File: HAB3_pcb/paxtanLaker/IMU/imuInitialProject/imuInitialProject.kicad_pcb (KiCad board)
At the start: 2 copper layers, 12 parts, among them J1 Conn_01x09_Female, J2 Conn_01x02_Female, U1 LSM9DS0

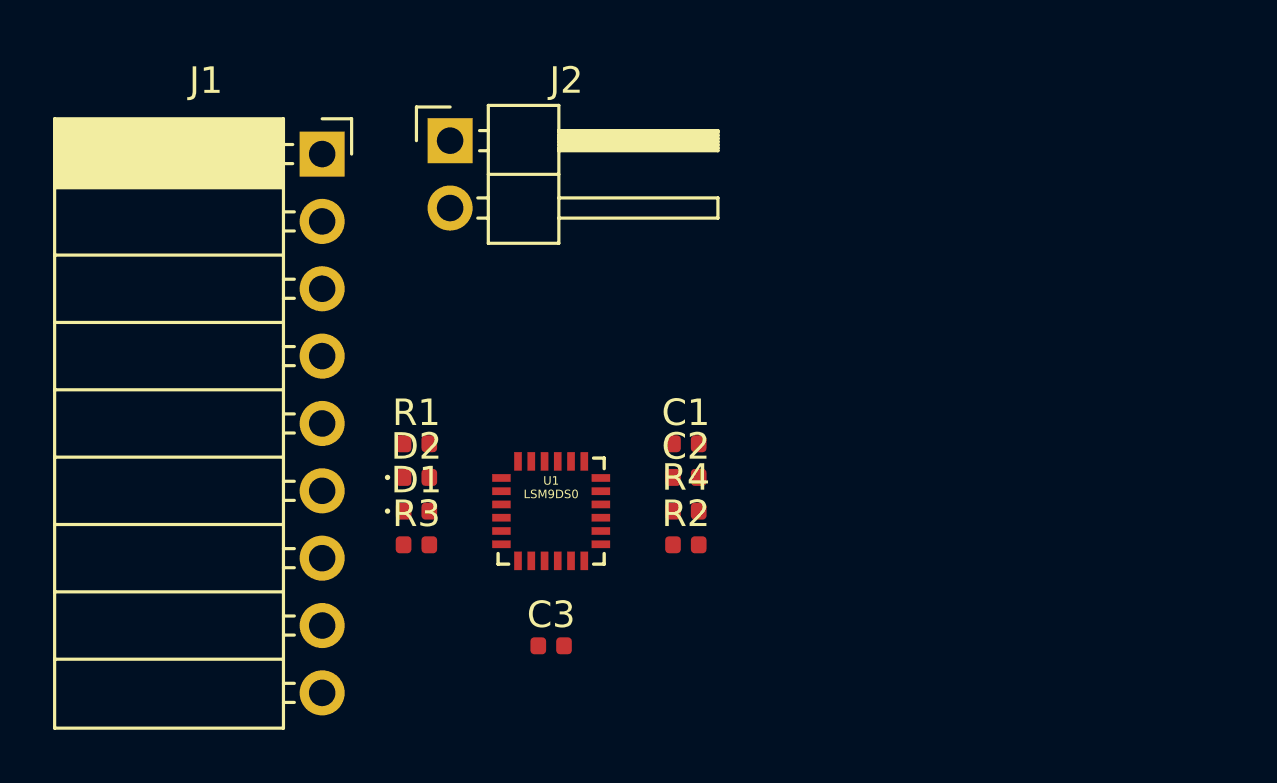
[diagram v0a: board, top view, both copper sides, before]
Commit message: started tracing
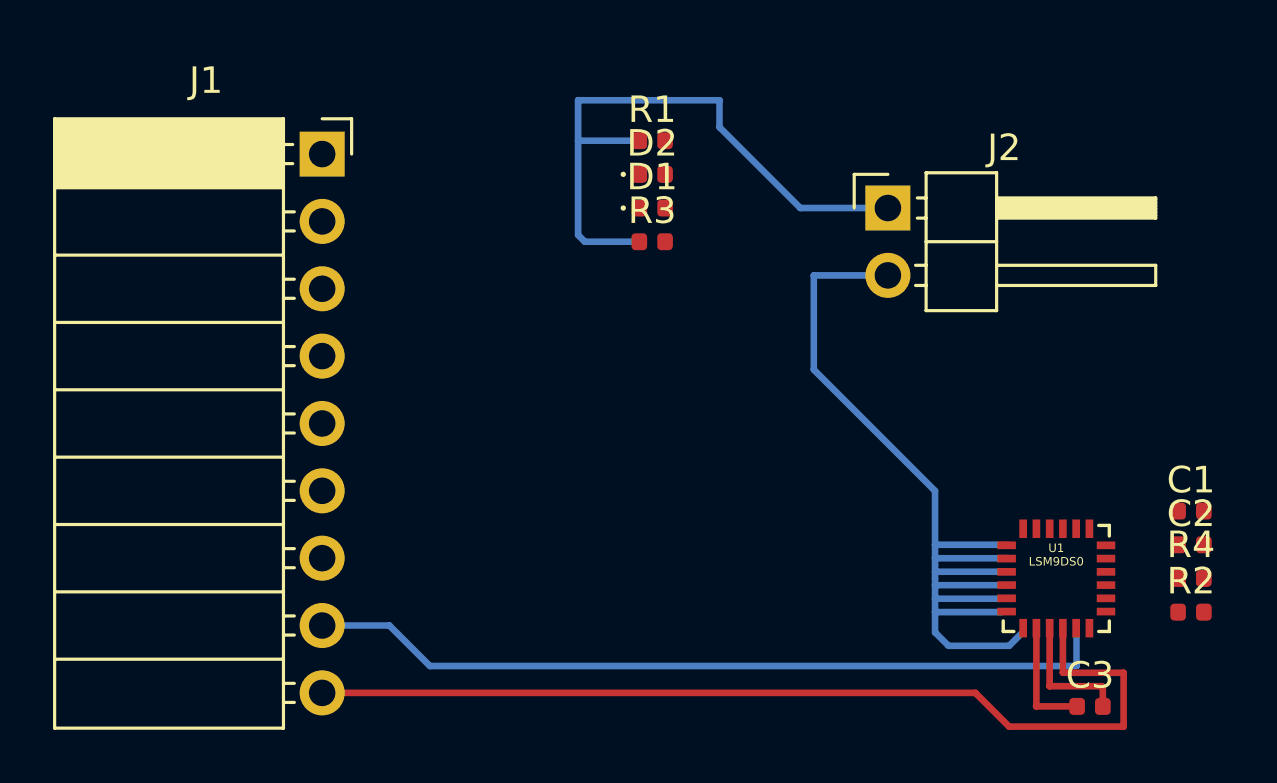
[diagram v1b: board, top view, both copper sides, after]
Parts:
- moved C3 20.4 mm to (167.6, 88.6)
- moved U1 19.2 mm to (166.4, 83.8)
- moved C1 19.2 mm to (171.4, 81.3)
- moved R2 19.2 mm to (171.4, 85.1)
- moved C2 19.2 mm to (171.4, 82.5)
- moved R4 19.2 mm to (171.4, 83.8)
- moved J2 16.7 mm to (160.0, 69.8)
- moved D1 14.5 mm to (151.1, 69.8)
- moved D2 14.5 mm to (151.1, 68.6)
- moved R1 14.5 mm to (151.1, 67.3)
- moved R3 14.5 mm to (151.1, 71.1)
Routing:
- net Net-(C1-Pad1): track 0.00 -> 38.1 mm
- net Net-(J1-Pad9): track 0.00 -> 36.8 mm
- net Net-(J1-Pad8): track 0.00 -> 30.3 mm
- net Net-(C1-Pad2): track 0.00 -> 23.7 mm
- net Net-(C3-Pad2): track 0.00 -> 4.95 mm
- net Net-(C3-Pad1): track 0.00 -> 4.50 mm
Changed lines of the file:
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@@
   (general
     (thickness 1.6)
-    (drawings 4)
-    (tracks 0)
+    (drawings 6)
+    (tracks 49)
     (zones 0)
     (modules 12)
@@
   )
   (module Capacitor_SMD:C_0402_1005Metric (layer F.Cu)
-    (at 152.4 78.74)
+    (at 171.45 81.28)
     (descr "Capacitor SMD 0402 (1005 Metric), square (rectangular) end terminal, IPC_7351 nominal, (Body size source: http://www.tortai-tech.com/upload/download/2011102023233369053.pdf), generated with kicad-footprint-generator")
     (tags capacitor)
@@
   )
   (module Capacitor_SMD:C_0402_1005Metric (layer F.Cu)
-    (at 152.4 80.01)
+    (at 171.45 82.55)
     (descr "Capacitor SMD 0402 (1005 Metric), square (rectangular) end terminal, IPC_7351 nominal, (Body size source: http://www.tortai-tech.com/upload/download/2011102023233369053.pdf), generated with kicad-footprint-generator")
     (tags capacitor)
@@
   )
   (module Capacitor_SMD:C_0402_1005Metric (layer F.Cu)
-    (at 147.32 86.36)
+    (at 167.64 88.646)
     (descr "Capacitor SMD 0402 (1005 Metric), square (rectangular) end terminal, IPC_7351 nominal, (Body size source: http://www.tortai-tech.com/upload/download/2011102023233369053.pdf), generated with kicad-footprint-generator")
     (tags capacitor)
@@
   )
   (module Diode_SMD:D_0402_1005Metric (layer F.Cu)
-    (at 142.24 81.28)
+    (at 151.13 69.85)
     (descr "Diode SMD 0402 (1005 Metric), square (rectangular) end terminal, IPC_7351 nominal, (Body size source: http://www.tortai-tech.com/upload/download/2011102023233369053.pdf), generated with kicad-footprint-generator")
     (tags diode)
@@
   )
   (module Diode_SMD:D_0402_1005Metric (layer F.Cu)
-    (at 142.24 80.01)
+    (at 151.13 68.58)
     (descr "Diode SMD 0402 (1005 Metric), square (rectangular) end terminal, IPC_7351 nominal, (Body size source: http://www.tortai-tech.com/upload/download/2011102023233369053.pdf), generated with kicad-footprint-generator")
     (tags diode)
@@
   )
   (module Resistor_SMD:R_0402_1005Metric (layer F.Cu)
-    (at 142.24 78.74)
+    (at 151.13 67.31)
     (descr "Resistor SMD 0402 (1005 Metric), square (rectangular) end terminal, IPC_7351 nominal, (Body size source: http://www.tortai-tech.com/upload/download/2011102023233369053.pdf), generated with kicad-footprint-generator")
     (tags resistor)
@@
   )
   (module Resistor_SMD:R_0402_1005Metric (layer F.Cu)
-    (at 152.4 82.55)
+    (at 171.45 85.09)
     (descr "Resistor SMD 0402 (1005 Metric), square (rectangular) end terminal, IPC_7351 nominal, (Body size source: http://www.tortai-tech.com/upload/download/2011102023233369053.pdf), generated with kicad-footprint-generator")
     (tags resistor)
@@
   )
   (module Resistor_SMD:R_0402_1005Metric (layer F.Cu)
-    (at 142.24 82.55)
+    (at 151.13 71.12)
     (descr "Resistor SMD 0402 (1005 Metric), square (rectangular) end terminal, IPC_7351 nominal, (Body size source: http://www.tortai-tech.com/upload/download/2011102023233369053.pdf), generated with kicad-footprint-generator")
     (tags resistor)
@@
   )
   (module Resistor_SMD:R_0402_1005Metric (layer F.Cu)
-    (at 152.4 81.28)
+    (at 171.45 83.82)
     (descr "Resistor SMD 0402 (1005 Metric), square (rectangular) end terminal, IPC_7351 nominal, (Body size source: http://www.tortai-tech.com/upload/download/2011102023233369053.pdf), generated with kicad-footprint-generator")
     (tags resistor)
@@
   )
   (module LSM9DS04:LGA-24LSM (layer F.Cu)
-    (at 147.32 81.28)
+    (at 166.37 83.82)
     (descr "<h3>LGA 4x4x1 mm 24-lead</h3><ul><li>0.5mm pitch</li><li>Pads are 0.35x0.2 mm square</li></ul><p>This package is used for:<p><ul><li>ST Micro LSM9DS0 3D accel/gyro/mag</li></ul>")
     (attr smd)
@@
   )
   (module Connector_PinHeader_2.54mm:PinHeader_1x02_P2.54mm_Horizontal (layer F.Cu)
-    (at 143.51 67.31)
+    (at 160.02 69.85)
     (descr "Through hole angled pin header, 1x02, 2.54mm pitch, 6mm pin length, single row")
     (tags "Through hole angled pin header THT 1x02 2.54mm single row")
@@
     (fp_line (start 10.55 4.35) (end 10.55 -1.8) (layer F.CrtYd) (width 0.05))
     (fp_line (start 10.55 -1.8) (end -1.8 -1.8) (layer F.CrtYd) (width 0.05))
-    (fp_text user %R (at 2.77 1.27 90) (layer F.Fab)
+    (fp_text user %R (at 2.54 1.27 90) (layer F.Fab)
       (effects (font (size 1 1) (thickness 0.15)))
     )
@@
     )
   )
+  (gr_line (start 176.53 64.77) (end 154.94 64.77) (angle 90) (layer F.Adhes) (width 0.2))
+  (gr_line (start 176.53 91.44) (end 176.53 64.77) (angle 90) (layer F.Adhes) (width 0.2))
+  (gr_line (start 154.94 91.44) (end 176.53 91.44) (angle 90) (layer F.Adhes) (width 0.2))
   (gr_line (start 154.94 64.77) (end 127 64.77) (angle 90) (layer F.Adhes) (width 0.2))
-  (gr_line (start 154.94 91.44) (end 154.94 64.77) (angle 90) (layer F.Adhes) (width 0.2))
   (gr_line (start 127 91.44) (end 154.94 91.44) (angle 90) (layer F.Adhes) (width 0.2))
   (gr_line (start 127 64.77) (end 127 91.44) (angle 90) (layer F.Adhes) (width 0.2))
+  (segment (start 167.155 88.646) (end 165.608 88.646) (width 0.25) (layer F.Cu) (net 1) (status 400000))
+  (segment (start 165.62 88.634) (end 165.62 85.695) (width 0.25) (layer F.Cu) (net 1) (status 800000))
+  (segment (start 165.608 88.646) (end 165.62 88.634) (width 0.25) (layer F.Cu) (net 1))
+  (segment (start 168.125 88.646) (end 168.125 87.907) (width 0.25) (layer F.Cu) (net 2) (status 400000))
+  (segment (start 166.12 87.88) (end 166.12 85.695) (width 0.25) (layer F.Cu) (net 2) (status 800000))
+  (segment (start 166.116 87.884) (end 166.12 87.88) (width 0.25) (layer F.Cu) (net 2))
+  (segment (start 168.102 87.884) (end 166.116 87.884) (width 0.25) (layer F.Cu) (net 2))
+  (segment (start 168.125 87.907) (end 168.102 87.884) (width 0.25) (layer F.Cu) (net 2))
+  (segment (start 138.685001 85.595001) (end 141.221001 85.595001) (width 0.25) (layer B.Cu) (net 12) (status 400000))
+  (segment (start 167.132 87.122) (end 167.132 85.852) (width 0.25) (layer B.Cu) (net 12))
+  (segment (start 142.748 87.122) (end 167.132 87.122) (width 0.25) (layer B.Cu) (net 12))
+  (segment (start 141.221001 85.595001) (end 142.748 87.122) (width 0.25) (layer B.Cu) (net 12))
+  (segment (start 166.62 85.695) (end 166.62 87.372) (width 0.25) (layer F.Cu) (net 13) (status 400000))
+  (segment (start 163.319001 88.135001) (end 138.685001 88.135001) (width 0.25) (layer F.Cu) (net 13) (status 800000))
+  (segment (start 164.592 89.408) (end 163.319001 88.135001) (width 0.25) (layer F.Cu) (net 13))
+  (segment (start 168.91 89.408) (end 164.592 89.408) (width 0.25) (layer F.Cu) (net 13))
+  (segment (start 168.91 87.376) (end 168.91 89.408) (width 0.25) (layer F.Cu) (net 13))
+  (segment (start 166.62 87.372) (end 166.624 87.376) (width 0.25) (layer F.Cu) (net 13))
+  (segment (start 166.624 87.376) (end 168.91 87.376) (width 0.25) (layer F.Cu) (net 13))
+  (segment (start 160.02 72.39) (end 157.226 72.39) (width 0.25) (layer B.Cu) (net 16) (status 400000))
+  (segment (start 164.592 86.36) (end 165.1 85.852) (width 0.25) (layer B.Cu) (net 16))
+  (segment (start 162.306 86.36) (end 164.592 86.36) (width 0.25) (layer B.Cu) (net 16))
+  (segment (start 161.798 85.852) (end 162.306 86.36) (width 0.25) (layer B.Cu) (net 16))
+  (segment (start 161.798 80.518) (end 161.798 82.55) (width 0.25) (layer B.Cu) (net 16))
+  (segment (start 161.798 82.55) (end 161.798 83.058) (width 0.25) (layer B.Cu) (net 16))
+  (segment (start 161.798 83.058) (end 161.798 83.312) (width 0.25) (layer B.Cu) (net 16))
+  (segment (start 161.798 83.312) (end 161.798 83.566) (width 0.25) (layer B.Cu) (net 16))
+  (segment (start 161.798 83.566) (end 161.798 83.82) (width 0.25) (layer B.Cu) (net 16))
+  (segment (start 161.798 83.82) (end 161.798 84.074) (width 0.25) (layer B.Cu) (net 16))
+  (segment (start 161.798 84.074) (end 161.798 84.582) (width 0.25) (layer B.Cu) (net 16))
+  (segment (start 161.798 84.582) (end 161.798 85.09) (width 0.25) (layer B.Cu) (net 16))
+  (segment (start 161.798 85.09) (end 161.798 85.852) (width 0.25) (layer B.Cu) (net 16))
+  (segment (start 157.226 75.946) (end 161.798 80.518) (width 0.25) (layer B.Cu) (net 16))
+  (segment (start 157.226 72.39) (end 157.226 75.946) (width 0.25) (layer B.Cu) (net 16))
+  (segment (start 161.798 85.09) (end 164.338 85.09) (width 0.25) (layer B.Cu) (net 16))
+  (segment (start 161.798 84.582) (end 164.592 84.582) (width 0.25) (layer B.Cu) (net 16))
+  (segment (start 161.798 84.074) (end 164.592 84.074) (width 0.25) (layer B.Cu) (net 16))
+  (segment (start 161.798 83.566) (end 164.338 83.566) (width 0.25) (layer B.Cu) (net 16))
+  (segment (start 161.798 83.058) (end 164.592 83.058) (width 0.25) (layer B.Cu) (net 16))
+  (segment (start 161.798 82.55) (end 164.592 82.55) (width 0.25) (layer B.Cu) (net 16))
+  (segment (start 160.02 69.85) (end 156.718 69.85) (width 0.25) (layer B.Cu) (net 17) (status 400000))
+  (segment (start 148.336 67.31) (end 150.622 67.31) (width 0.25) (layer B.Cu) (net 17))
+  (segment (start 148.336 65.786) (end 148.336 67.31) (width 0.25) (layer B.Cu) (net 17))
+  (segment (start 153.67 65.786) (end 148.336 65.786) (width 0.25) (layer B.Cu) (net 17))
+  (segment (start 156.718 69.85) (end 153.67 66.802) (width 0.25) (layer B.Cu) (net 17))
+  (segment (start 153.67 66.802) (end 153.67 65.786) (width 0.25) (layer B.Cu) (net 17))
+  (segment (start 148.336 67.31) (end 148.336 70.866) (width 0.25) (layer B.Cu) (net 17))
+  (segment (start 148.59 71.12) (end 150.622 71.12) (width 0.25) (layer B.Cu) (net 17))
+  (segment (start 148.336 70.866) (end 148.59 71.12) (width 0.25) (layer B.Cu) (net 17))
 )
